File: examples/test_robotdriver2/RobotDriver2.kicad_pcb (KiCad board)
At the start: 2 copper layers, 125 x 75 mm, 68 parts, among them J1 C64658, J3 C265088, J4 C265088, J6 C64658, J7 C64658, J8 C64658, J9 C64658, SW1 C318884, U1 C7972, U2 C500769, U3 C701342, U4 C967633, U5 C50506, U6 C50506

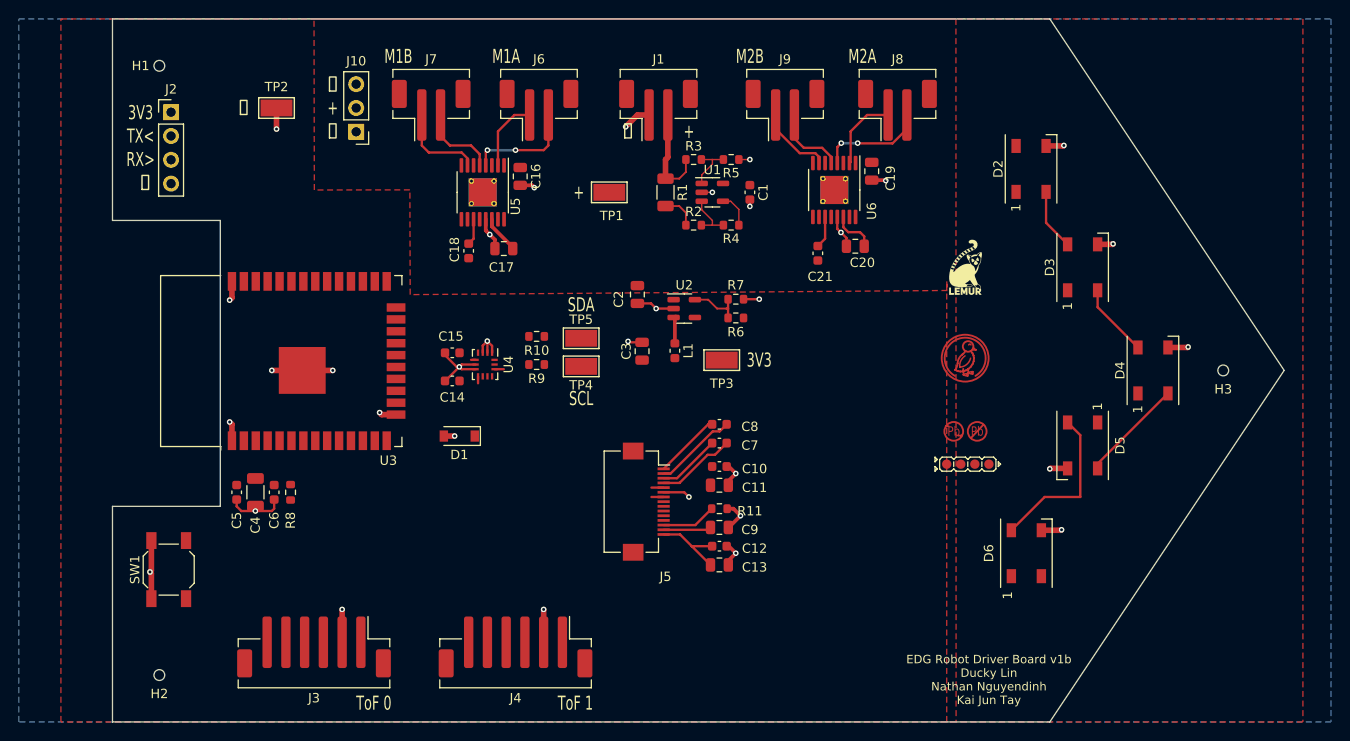
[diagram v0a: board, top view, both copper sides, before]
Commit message: cleanup for routing
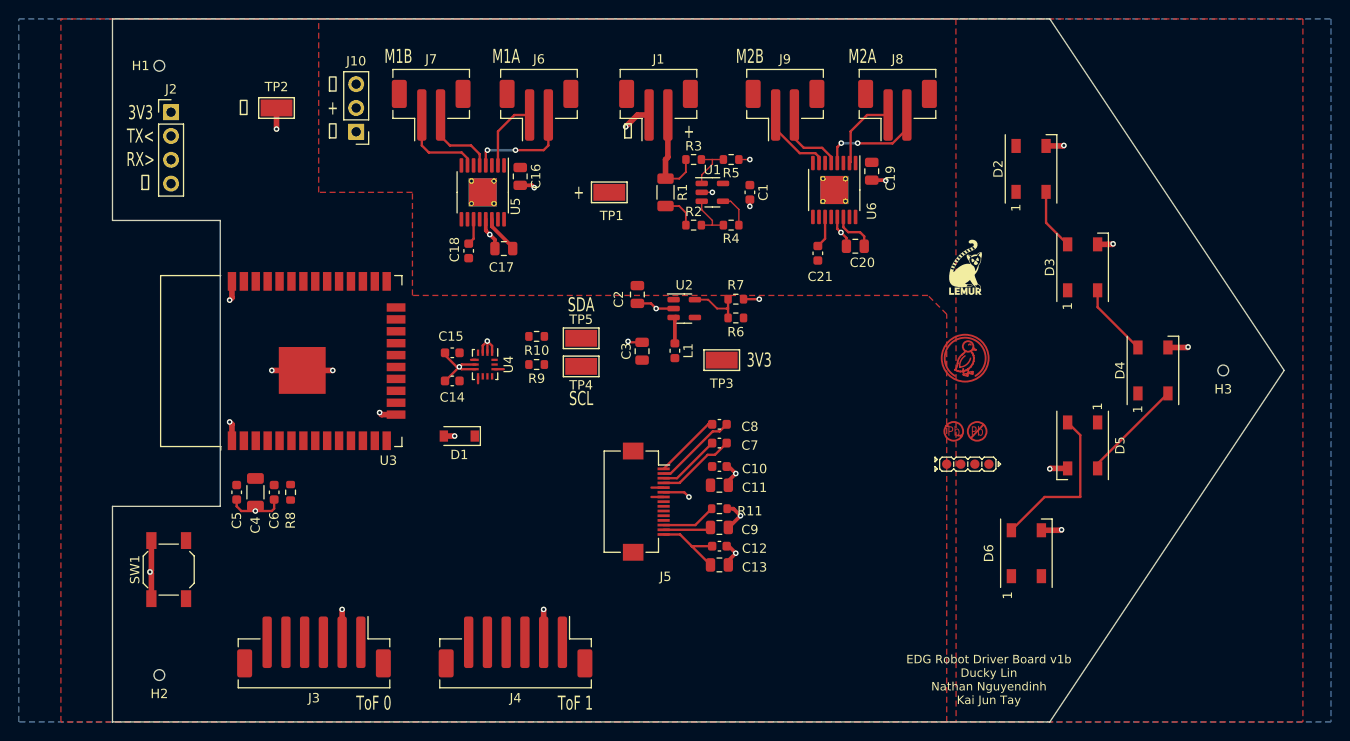
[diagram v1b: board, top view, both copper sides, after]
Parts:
- renumbered 2 to U10, 1 to U9
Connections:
- net isense.amp.amp.inn renamed isense.amp.(adapter)r1.b.src
- net isense.amp.amp.inp renamed isense.amp.r2.b
- net lcd.c2_cap.pos renamed lcd.device.c2p
- net lcd.iref_res.a renamed lcd.device.iref
- net mcu.ic.chip_pu renamed mcu.en_pull.output
- net mcu.ic.io0 renamed mcu.prog.out
- net motor_driver1.vcp_cap.pos renamed motor_driver1.ic.vcp
- net motor_driver1.vint_cap.pos renamed motor_driver1.vint_cap.pwr
- net reg_3v3.ic.fb renamed reg_3v3.fb.center
